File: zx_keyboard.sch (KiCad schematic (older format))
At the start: 62 parts, among them P1 CONN_02X08, SW1 KEY_1, SW10 KEY_0, SW11 KEY_Q, SW12 KEY_W, SW13 KEY_E, SW14 KEY_R, SW15 KEY_T, SW16 KEY_Y, SW17 KEY_U, SW18 KEY_I, SW19 KEY_O, SW2 KEY_2, SW20 KEY_P, SW21 KEY_A, SW22 KEY_S, SW23 KEY_D, SW24 KEY_F, SW25 KEY_G, SW26 KEY_H, SW27 KEY_J, SW28 KEY_K, SW29 KEY_L, SW3 KEY_3, SW30 KEY_EN, SW31 KEY_CS1, SW32 KEY_Z, SW33 KEY_X, SW34 KEY_C, SW35 KEY_V, SW36 KEY_B, SW37 KEY_N, SW38 KEY_M, SW39 KEY_SS1, SW4 KEY_4, SW40 KEY_SP, SW41 KEY_CS2, SW42 KEY_SS2, SW43 KEY_TV, SW5 KEY_5, SW6 KEY_6, SW7 KEY_7, SW8 KEY_8, SW9 KEY_9, U1 4066

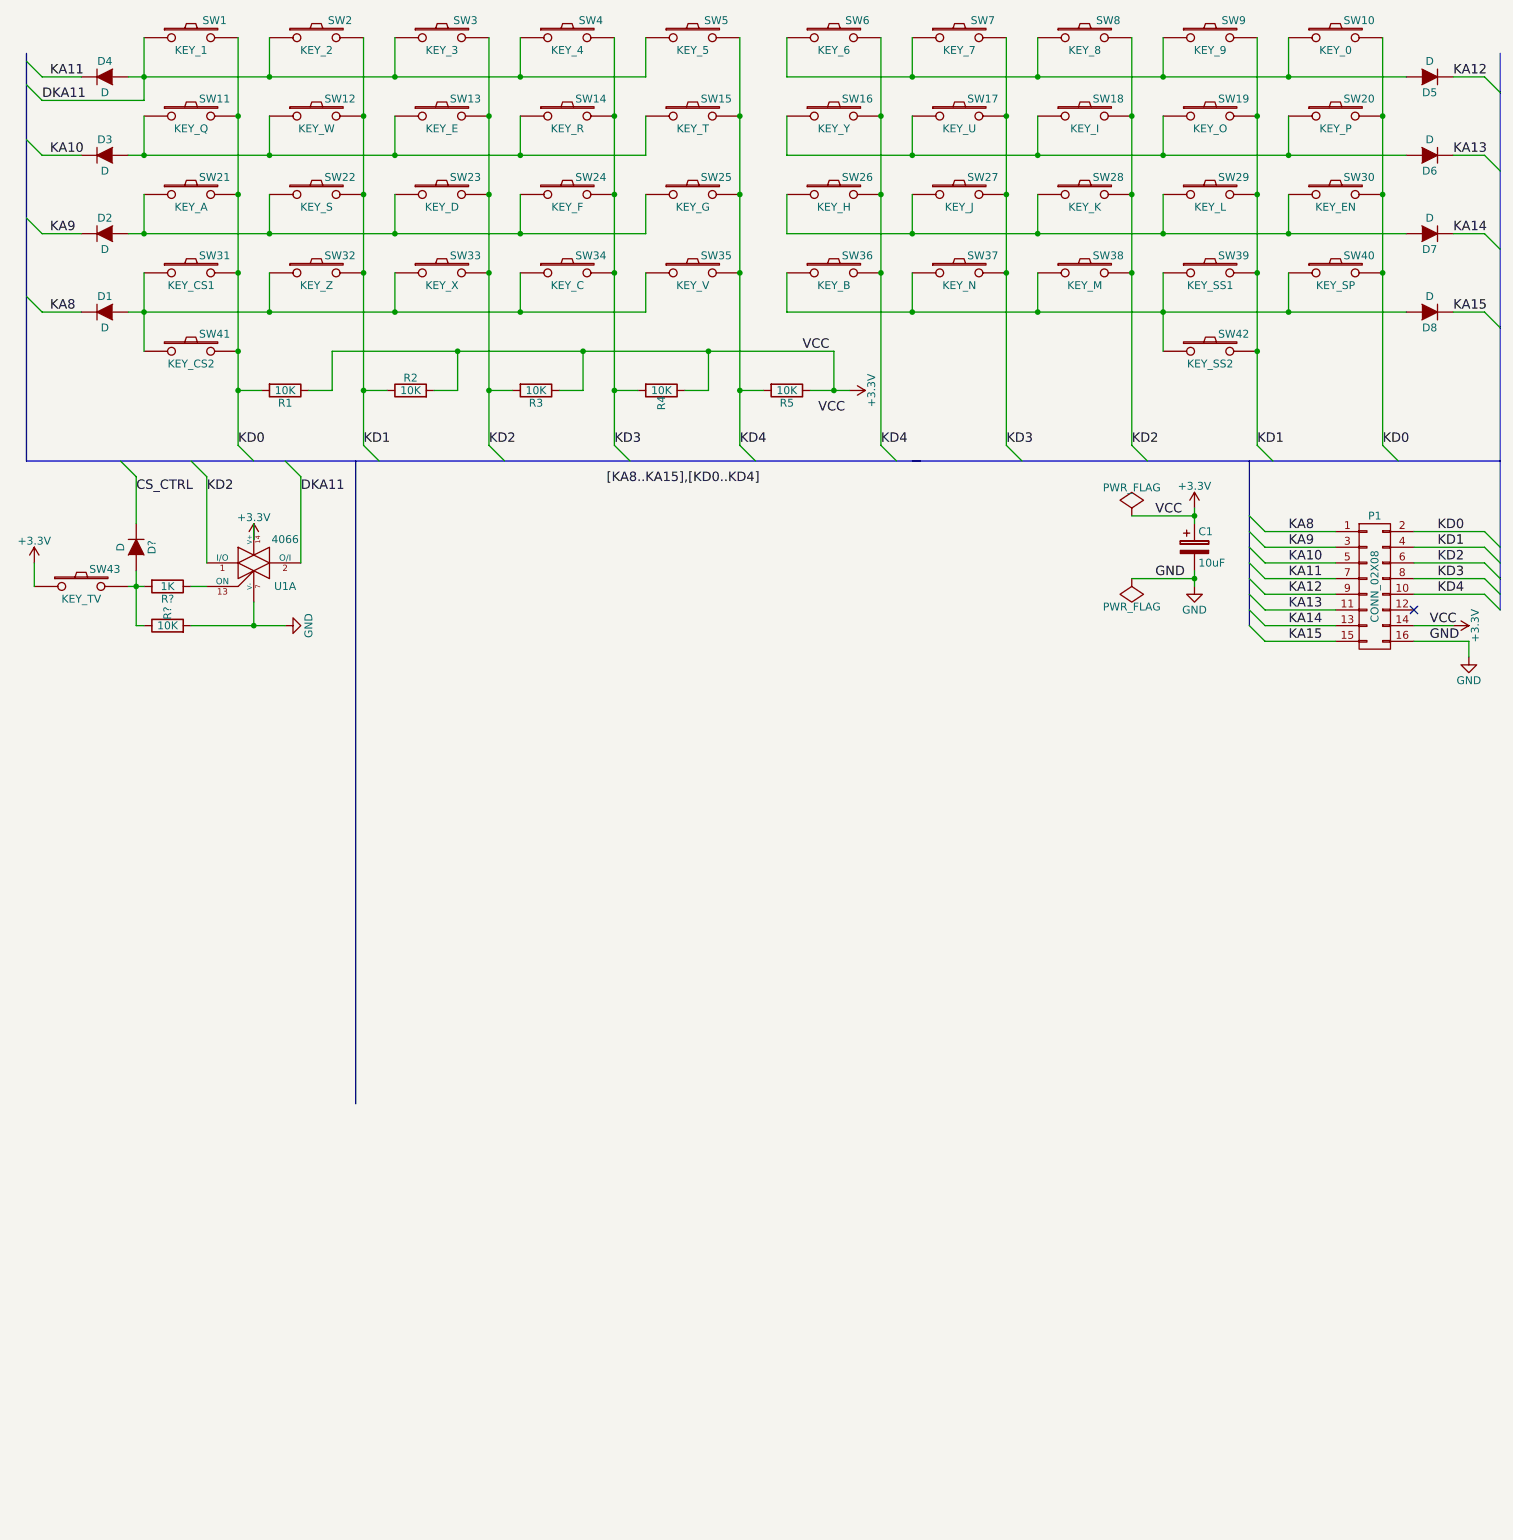
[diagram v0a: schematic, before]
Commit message: zx
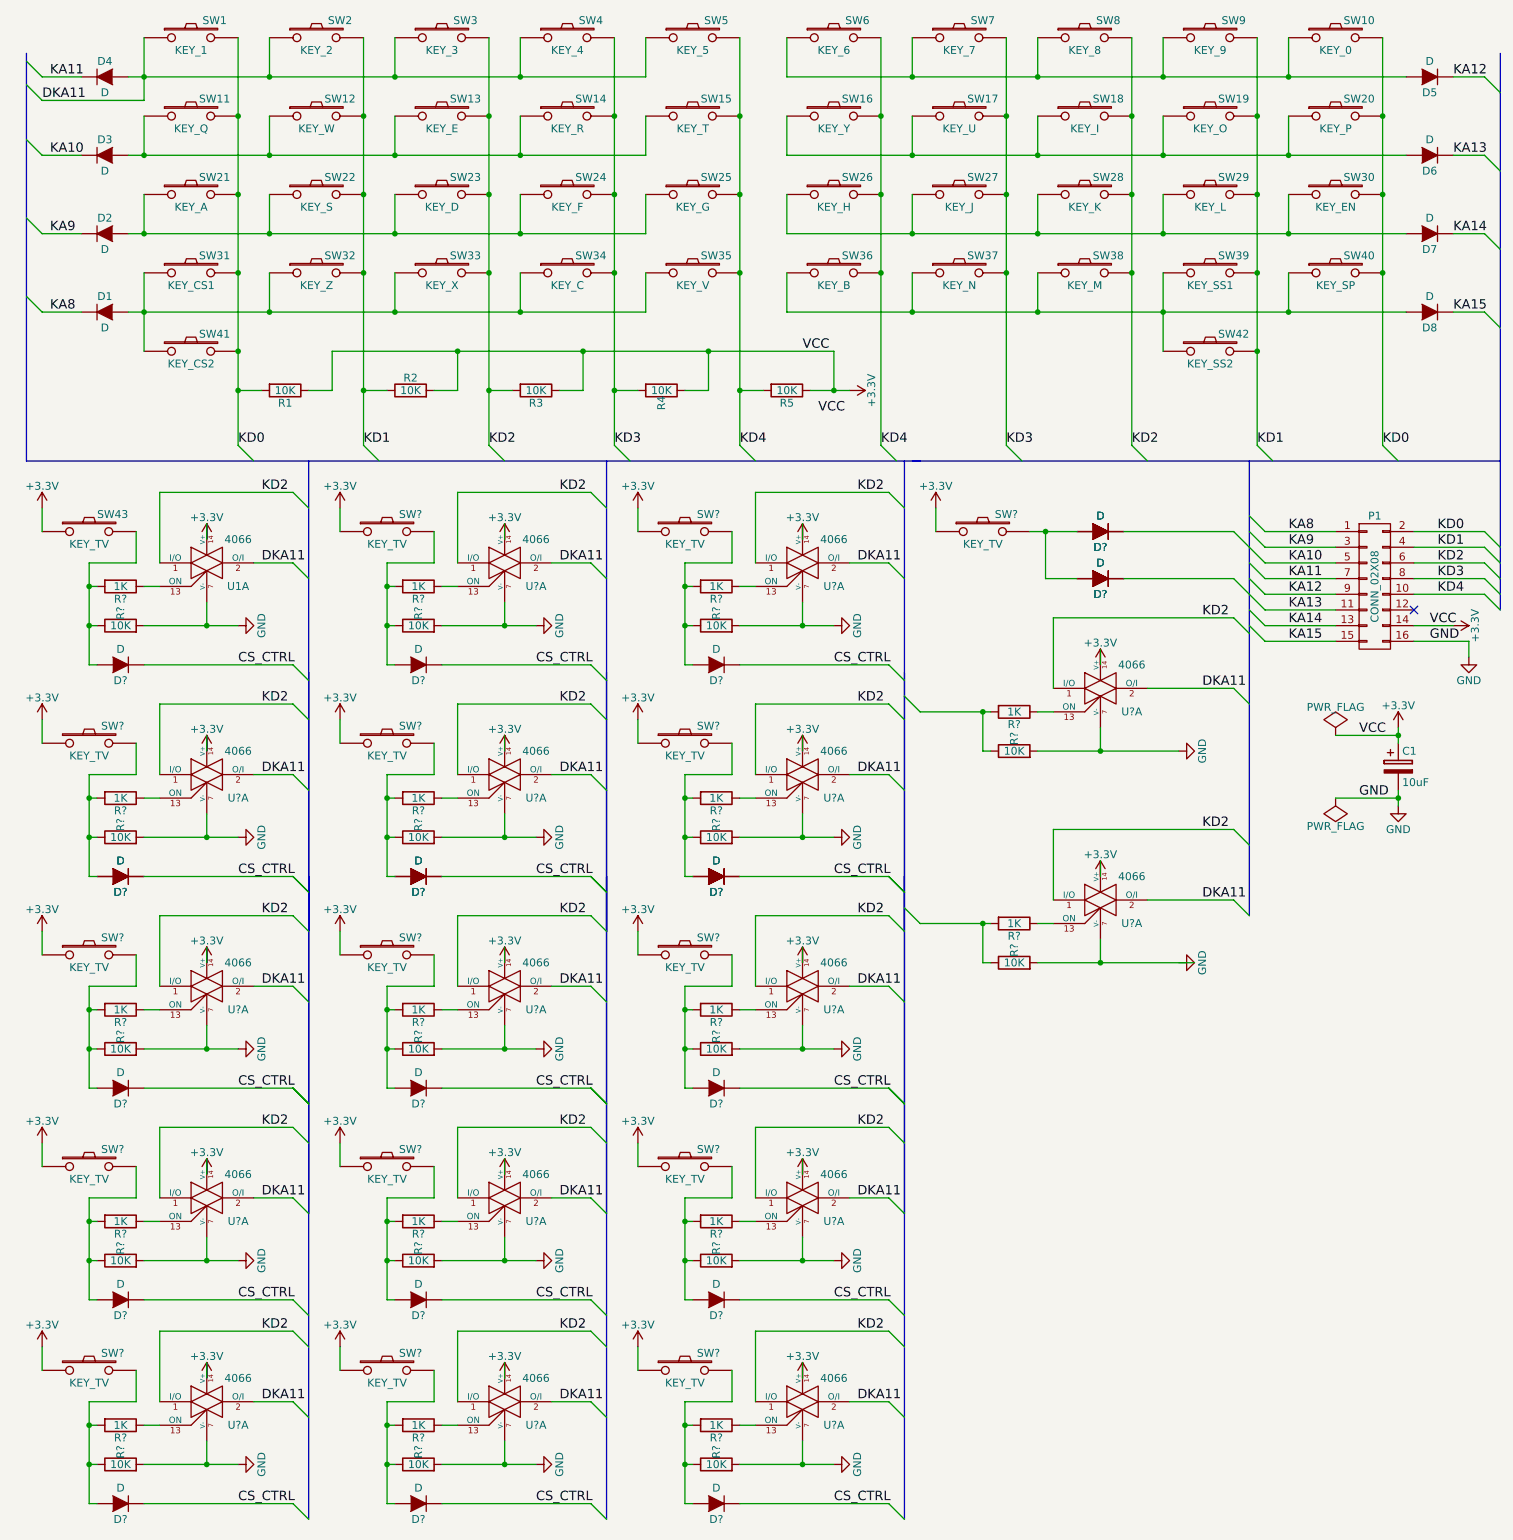
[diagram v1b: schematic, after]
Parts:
- added D? (x21): D, symbol D
- added R? (x16): 1K, symbol R
- added R? (x16): 10K, symbol R
- added SW? (x15): KEY_TV, Buttons_Switches_Keyboard:SW_Cherry_MX1A_1.00u_PCB, symbol SW_PUSH
- added U? (x16): 4066, TO_SOT_Packages_SMD:SOT-428, symbol 4066
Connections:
- net +3V3: now also SW?.1, SW?.1, SW?.1, SW?.1, SW?.1, SW?.1, SW?.1, SW?.1, SW?.1, SW?.1, SW?.1, SW?.1, SW?.1, SW?.1, SW?.1, U?.14 (V+), U?.14 (V+), U?.14 (V+), U?.14 (V+), U?.14 (V+), U?.14 (V+), U?.14 (V+), U?.14 (V+), U?.14 (V+), U?.14 (V+), U?.14 (V+), U?.14 (V+), U?.14 (V+), U?.14 (V+), U?.14 (V+), U?.14 (V+)
- net CS_CTRL: now also D?.1 (K), D?.1 (K), D?.1 (K), D?.1 (K), D?.1 (K), D?.1 (K), D?.1 (K), D?.1 (K), D?.1 (K), D?.1 (K), D?.1 (K), D?.1 (K), D?.1 (K), D?.1 (K), D?.1 (K), D?.1 (K), D?.1 (K)
- net DKA11: now also U?.2 (O/I), U?.2 (O/I), U?.2 (O/I), U?.2 (O/I), U?.2 (O/I), U?.2 (O/I), U?.2 (O/I), U?.2 (O/I), U?.2 (O/I), U?.2 (O/I), U?.2 (O/I), U?.2 (O/I), U?.2 (O/I), U?.2 (O/I), U?.2 (O/I), U?.2 (O/I)
- net GND: now also R?.2, R?.2, R?.2, R?.2, R?.2, R?.2, R?.2, R?.2, R?.2, R?.2, R?.2, R?.2, R?.2, R?.2, R?.2, U?.7 (V-), U?.7 (V-), U?.7 (V-), U?.7 (V-), U?.7 (V-), U?.7 (V-), U?.7 (V-), U?.7 (V-), U?.7 (V-), U?.7 (V-), U?.7 (V-), U?.7 (V-), U?.7 (V-), U?.7 (V-), U?.7 (V-)
- net KD2: now also U?.1 (I/O), U?.1 (I/O), U?.1 (I/O), U?.1 (I/O), U?.1 (I/O), U?.1 (I/O), U?.1 (I/O), U?.1 (I/O), U?.1 (I/O), U?.1 (I/O), U?.1 (I/O), U?.1 (I/O), U?.1 (I/O), U?.1 (I/O), U?.1 (I/O), U?.1 (I/O)
- new net: R?.1, U?.13 (ON) (x16)
- new net: D?.2 (A), D?.2 (A), R?.1, R?.2, SW?.2 (x3)
- new net: D?.2 (A), R?.1, R?.2, SW?.2 (x11)
- new net: D?.2 (A), D?.2 (A), D?.2 (A), D?.2 (A), SW?.2
- new net: R?.1, R?.2 (x2)
- new net: D?.1 (K), D?.1 (K) (x2)
- new net: R?.2, U?.7 (V-)
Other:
- moved on the sheet: C1, D?, R?, SW43, U1A
